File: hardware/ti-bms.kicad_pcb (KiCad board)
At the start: 2 copper layers, 93.5 x 53 mm, 64 parts, among them J1 Conn_02x03_Odd_Even, J2 Conn_01x02, J3 Conn_01x02, J4 Conn_01x02, J5 CAN_TERM, U1 Pico, U2 MCP2515-xST, U3 SN65HVD230, U4 TPS62160DGK, U5 MAX3485, U6 MAX3485, U7 MAX3485

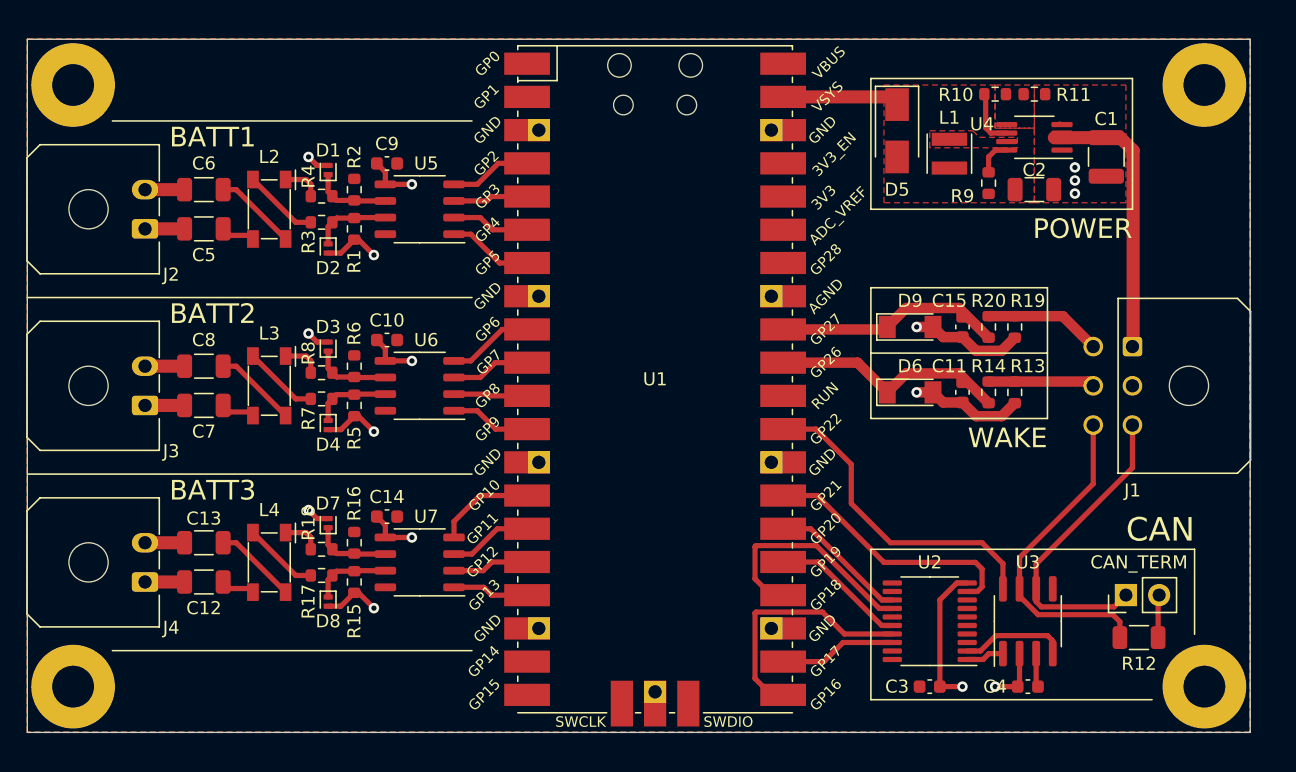
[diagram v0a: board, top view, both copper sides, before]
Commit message: merge v3 improvements into v2
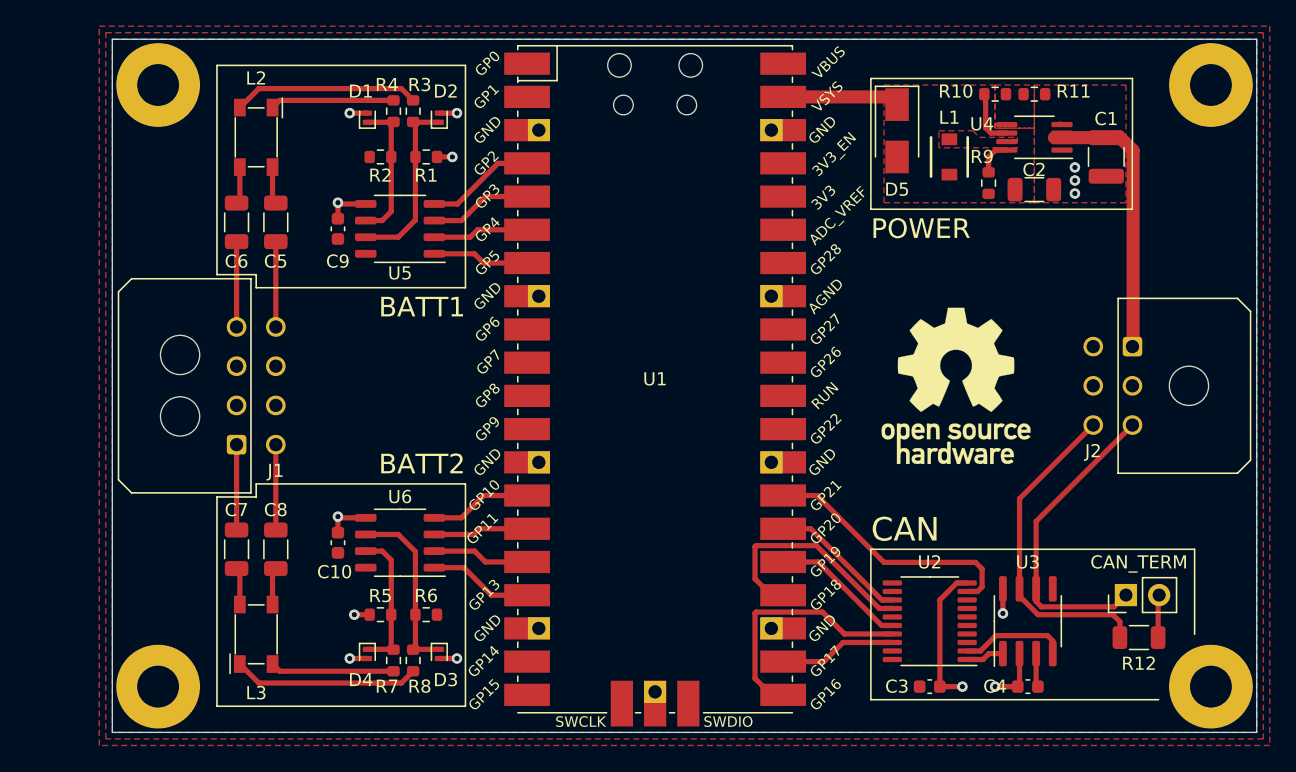
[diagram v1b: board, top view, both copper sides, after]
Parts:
- removed C11, C14, C15: 100n, Capacitor_SMD:C_0603_1608Metric
- removed C12, C13: 1n 1000v, Capacitor_SMD:C_1206_3216Metric
- removed D6, D9: 3.3v, Diode_SMD:D_MiniMELF
- removed D7, D8: 5v, footprints:SOD882
- removed J3: Conn_01x02, Connector_Molex:Molex_Micro-Fit_3.0_43650-0200_1x02_P3.00mm_Horizontal
- removed the J4 at (91.5, 103.5)
- removed L4: 22u, footprints:ACT45B-101-2P-TL003
- removed R13, R19: 47k, Resistor_SMD:R_0603_1608Metric
- removed R14, R20: 5.6k, Resistor_SMD:R_0603_1608Metric
- removed R15, R16: 1k, Resistor_SMD:R_0603_1608Metric
- removed R17, R18: 10, Resistor_SMD:R_0603_1608Metric
- removed U7: MAX3485, Package_SO:SOP-8_3.9x4.9mm_P1.27mm
- added REF**: OSHW-Logo_11.4x12mm_SilkScreen, Symbol:OSHW-Logo_11.4x12mm_SilkScreen, F.Cu at (153.5, 88.5)
- J1: value Conn_02x03_Odd_Even -> Conn_02x04_Odd_Even; footprint Connector_Molex:Molex_Micro-Fit_3.0_43045-0600_2x03_P3.00mm_Horizontal -> Connector_Molex:Molex_Micro-Fit_3.0_43045-0800_2x04_P3.00mm_Horizontal
- J2: value Conn_01x02 -> Conn_02x03_Odd_Even; footprint Connector_Molex:Molex_Micro-Fit_3.0_43650-0200_1x02_P3.00mm_Horizontal -> Connector_Molex:Molex_Micro-Fit_3.0_43045-0600_2x03_P3.00mm_Horizontal
- L1: footprint Inductor_SMD:L_Neosid_SMS-ME3015 -> footprints:1227ASH100MP2
- moved J2 76.0 mm to (167.0, 85.5), turned to 270 degrees
- moved J1 68.9 mm to (98.5, 93.0), turned to 90 degrees
- moved D3 25.0 mm to (114.0, 109.0), turned to 270 degrees
- moved R8 23.1 mm to (112.0, 109.5), turned to 90 degrees
- moved R7 20.7 mm to (110.5, 109.5), turned to 90 degrees
- moved R6 19.8 mm to (113.0, 106.0), turned to 0 degrees
- moved L3 19.0 mm to (100.0, 107.5), turned to 90 degrees
- moved D4 17.8 mm to (108.5, 109.0)
- moved R5 16.1 mm to (109.5, 106.0), turned to 0 degrees
- moved C10 15.9 mm to (106.2, 100.5), turned to 90 degrees
- moved C8 15.0 mm to (101.5, 101.0), turned to 270 degrees
- moved D2 13.1 mm to (114.0, 68.0), turned to 90 degrees
- moved U6 12.1 mm to (111.0, 100.5)
- moved C7 11.3 mm to (98.5, 101.0), turned to 270 degrees
- moved R3 11.0 mm to (112.0, 67.5), turned to 270 degrees
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- renumbered J5 to J4
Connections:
- C5 pad 1: B1- -> B1+
- C6 pad 1: B1+ -> B1-
- C7 pad 1: B2- -> B2+
- C8 pad 1: B2+ -> B2-
- J1 pad 1: +12V -> B2+
- J1 pad 2: GND -> (no net)
- J1 pad 3: CANL -> (no net)
- J1 pad 4: WAKE2 -> B1-
- J1 pad 5: WAKE1 -> B2-
- J1 pad 6: CANH -> (no net)
- J2 pad 1: B1- -> +12V
- J2 pad 2: B1+ -> GND
- L2 pad 3: Net-(C6-Pad2) -> Net-(C5-Pad2)
- L2 pad 4: Net-(C5-Pad2) -> Net-(C6-Pad2)
- L3 pad 3: Net-(C8-Pad2) -> Net-(C7-Pad2)
- L3 pad 4: Net-(C7-Pad2) -> Net-(C8-Pad2)
- U1 pad 10: TXE_2 -> (no net)
- U1 pad 11: RXE_2 -> (no net)
- U1 pad 12: RXD_2 -> (no net)
- U1 pad 14: TXD_3 -> TXD_2
- U1 pad 15: TXE_3 -> TXE_2
- U1 pad 16: RXE_3 -> RXE_2
- U1 pad 17: RXD_3 -> RXD_2
- U1 pad 29: Rs -> (no net)
- U1 pad 31: IN1 -> (no net)
- U1 pad 32: IN2 -> (no net)
- U1 pad 9: TXD_2 -> (no net)
- U3 pad 8: Rs -> GND
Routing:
- net GND: track 62.9 -> 31.7 mm, vias 16 -> 14
- net Rs: track 25.7 -> 0.00 mm
- net IN1: track 19.1 -> 0.00 mm
- net IN2: track 18.2 -> 0.00 mm
- net Net-(L3-Pad1): track 2.99 -> 14.2 mm
- net WAKE2: track 8.96 -> 0.00 mm
- net TXD_3: track 8.53 -> 0.00 mm
- net Net-(L2-Pad2): track 5.78 -> 14.2 mm
- net WAKE1: track 8.13 -> 0.00 mm
- net Net-(D3-Pad1): track 5.99 -> 13.9 mm
- net Net-(D2-Pad1): track 5.99 -> 13.9 mm
- net TXE_3: track 7.29 -> 0.00 mm
- net RXE_3: track 6.76 -> 0.00 mm
- net RXD_3: track 6.74 -> 0.00 mm
- net Net-(L2-Pad1): track 2.99 -> 9.48 mm
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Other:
- board size 93.5 x 53 mm -> 87.5 x 53 mm
- net class HV added: clearance 1.5, trace_width 0.25, via_dia 0.8, via_drill 0.4
- board text removed: "BATT3"
- board text removed: "Daisychain BMS v3"
- board text removed: "WAKE"
